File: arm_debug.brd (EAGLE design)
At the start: 40.3 x 19 mm, 11 parts

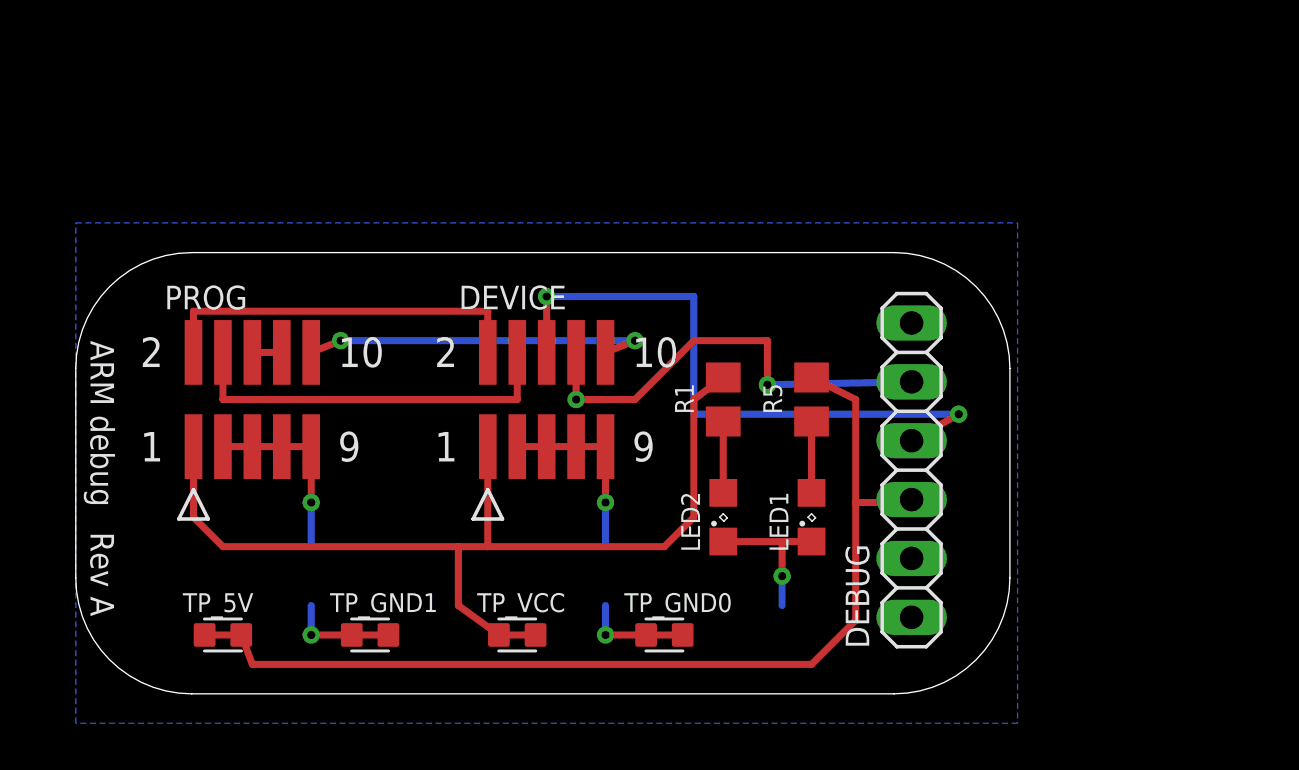
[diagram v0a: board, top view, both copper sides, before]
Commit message: Saving place.. currently working on Rev B
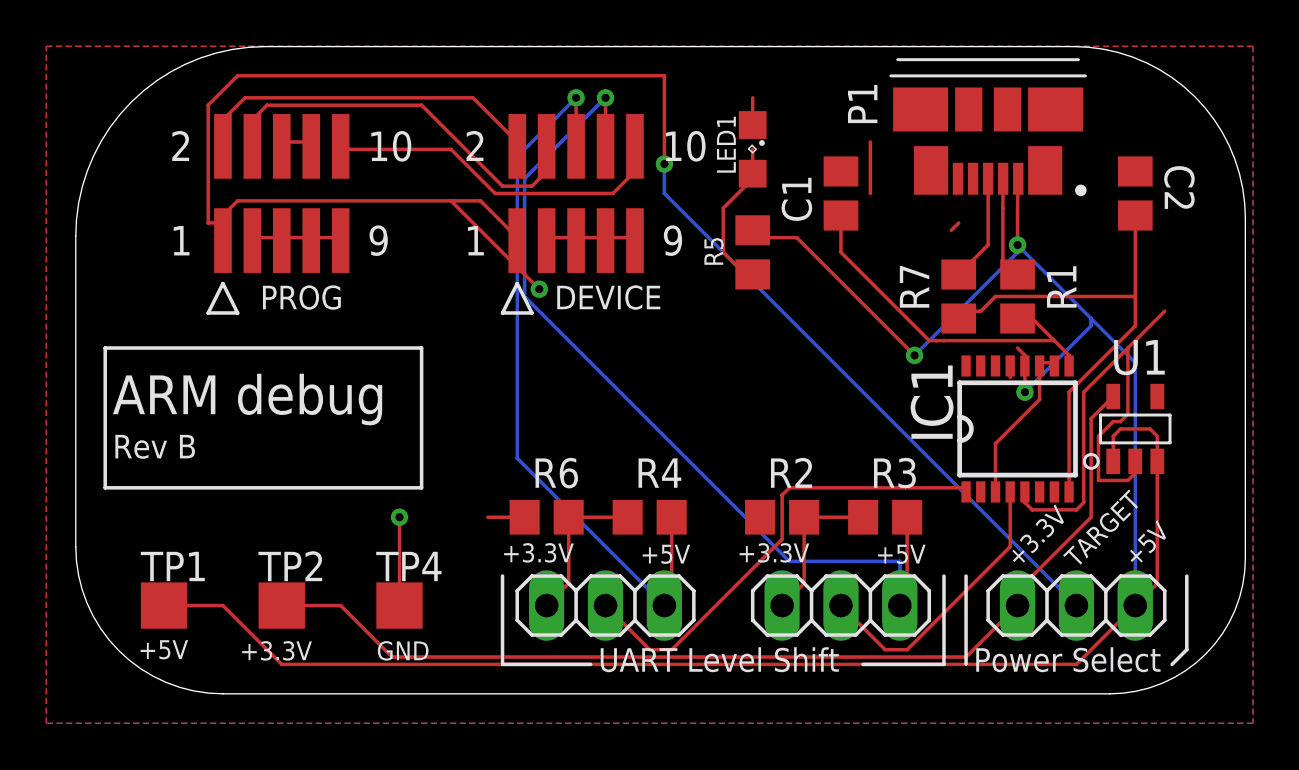
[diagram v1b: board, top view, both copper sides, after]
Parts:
- removed DEBUG: (no value), pinhead:1X06
- removed LED2: (no value), led:SML0805
- removed TP_5V, TP_GND0, TP_GND1, TP_VCC: 1625854-3, 1625854-3:RESC1608X50N
- added C1, C2: (no value), resistor:C0805
- added IC1: FT230XSS, FT230XS:SSOP16
- added JP1, JP2, PWR_SELECT: (no value), pinhead:1X03
- added P1: 0473460001, 0473460001:MOLEX_0473460001
- added R2, R3, R4, R6, R7: (no value), resistor:R0805
- added TP1, TP2, TP4: TPTP20SQ, testpad:TP20SQ
- added U1: CAT6219, CAT6219-330TDGT3:SOT-23(OT)5_LEAD
- moved LED1 16.1 mm to (29.2, 23.5), turned to 270 degrees
- moved R1 13.5 mm to (40.6, 17.1)
- moved DEVICE 8.98 mm to (21.6, 21.6)
- moved PROG 8.98 mm to (8.89, 21.6)
- moved R5 6.84 mm to (29.2, 19.1)
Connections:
- removed net !CTS: DEBUG.2
- removed net !RTS: DEBUG.6
- removed net VCC: DEVICE.1, PROG.1, R1.2, TP_VCC.1, TP_VCC.2
- new net +3V3: PWR_SELECT.3, TP2.TP, U1.5
- new net D+: C2.1, IC1.8, R7.1
- new net D-: C1.1, IC1.9, R1.1
- new net FT230_RX: IC1.4, JP1.2
- new net FT230_TX: IC1.1, JP2.2
- new net N$3: IC1.10, IC1.11, IC1.3
- new net N$4: P1.3, R7.2
- new net N$7: JP2.3, R4.1, R6.2
- new net N$8: JP1.3, R2.2, R3.1
- new net TARGET_PWR: DEVICE.1, PROG.1, PWR_SELECT.2
- net +5V: now also IC1.12, P1.1, PWR_SELECT.1, TP1.TP, U1.1, U1.3; no longer DEBUG.3, TP_5V.1, TP_5V.2
- net DEBUG_UART_RX: now also JP2.1, R4.2; no longer DEBUG.4
- net DEBUG_UART_TX: now also JP1.1, R3.2; no longer DEBUG.5
- net GND: now also C1.2, C2.2, IC1.13, IC1.5, P1.5, R2.1, R6.1, TP4.TP, U1.2; no longer DEBUG.1, LED2.C, TP_GND0.1, TP_GND0.2, TP_GND1.1, TP_GND1.2
- net N$2: now also P1.2, R1.2; no longer LED2.A, R1.1
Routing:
- net TARGET_PWR: track 0.00 -> 76.4 mm, vias 0 -> 2
- net +5V: track 43.8 -> 97.9 mm, vias 0 -> 3
- net +3V3: track 0.00 -> 44.3 mm
- net VCC: track 43.0 -> 0.00 mm
- net D+: track 0.00 -> 21.3 mm
- net FT230_TX: track 0.00 -> 20.5 mm
- net DEBUG_UART_TX: track 19.5 -> 38.9 mm, vias 2 -> 1
- net D-: track 0.00 -> 15.7 mm
- net FT230_RX: track 0.00 -> 12.3 mm
- net GND: track 32.0 -> 41.4 mm, vias 5 -> 1
- net N$3: track 0.00 -> 7.14 mm
- net N$8: track 0.00 -> 6.75 mm
- net N$7: track 0.00 -> 6.75 mm
- net N$4: track 0.00 -> 4.98 mm
- net DEBUG_UART_RX: track 27.6 -> 31.6 mm, vias 2 -> 1
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- added copper zone on layer 1, net GND
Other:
- board size 40.3 x 19 mm -> 50.5 x 27.9 mm
- board text added: "+3.3V"
- board text added: "+5V"
- board text added: "GND"
- board text added: "Power Select"
- board text added: "Rev B"
- board text added: "TARGET"
- board text added: "UART Level Shift"
- board text removed: "Rev A"
